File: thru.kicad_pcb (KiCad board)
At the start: 2 copper layers, 33.3 x 12.3 mm, 2 parts, among them J2 Conn_Coaxial, J4 Conn_Coaxial

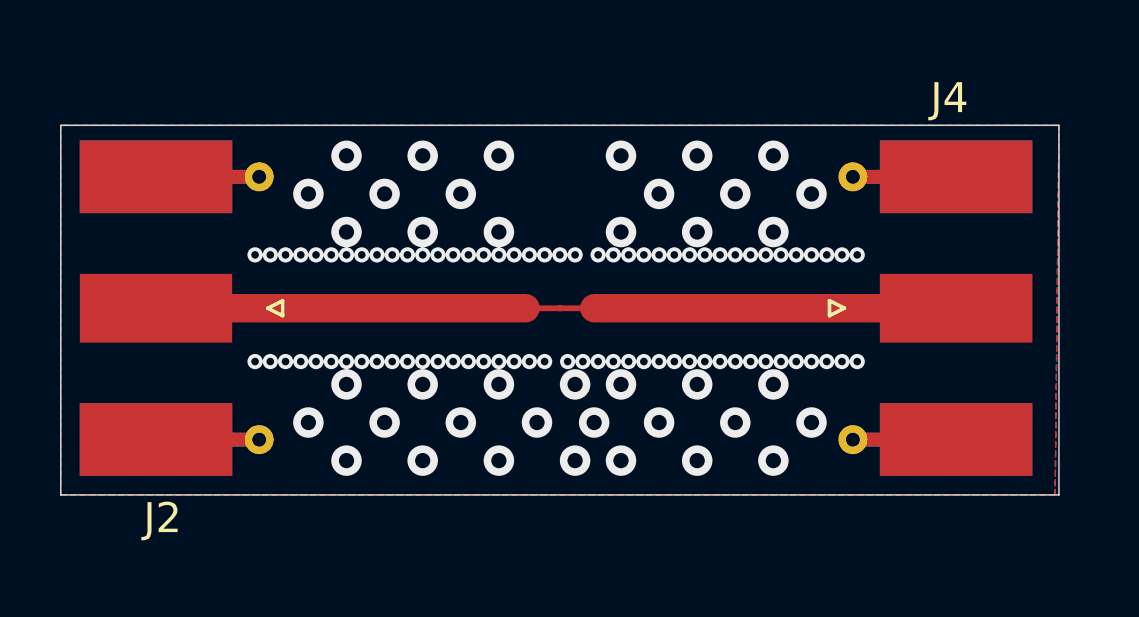
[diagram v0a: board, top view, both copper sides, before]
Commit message: made a southwest microwave launch and put it in the thru
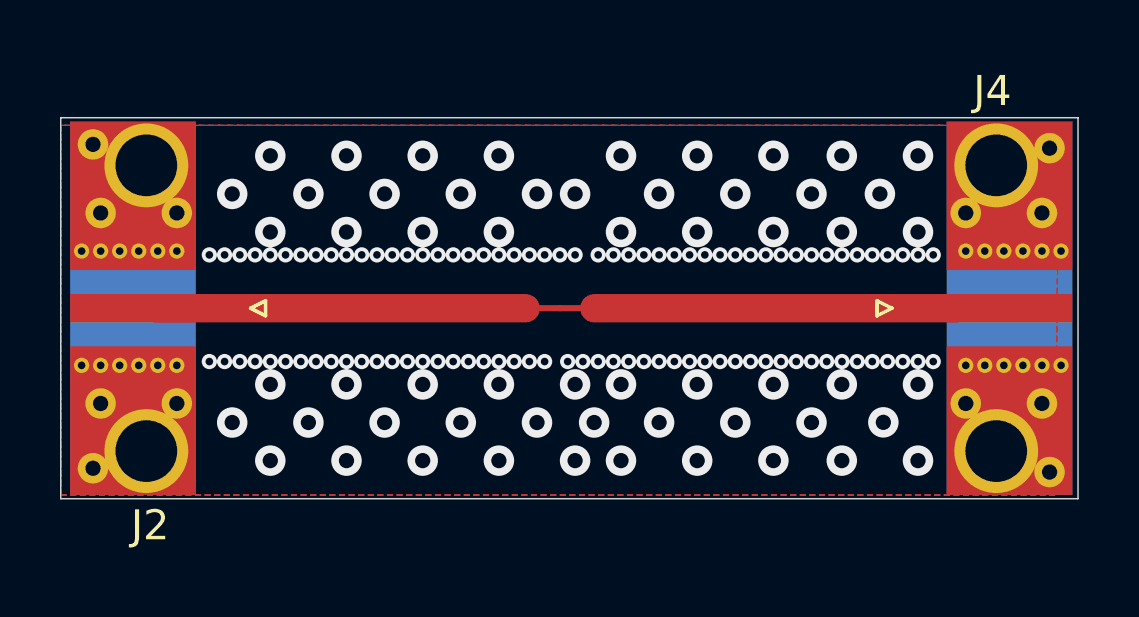
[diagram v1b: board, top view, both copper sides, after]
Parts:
- J2, J4: footprint Connector_Coaxial:SMA_Molex_73251-1153_EdgeMount_Horizontal -> southwest-microwave-connectors:southwest-super-SMA-292-04A-12
- moved J4 5.85 mm to (184.0, 125.4)
- moved J2 4.84 mm to (150.1, 125.4)
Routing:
- net GND: vias 120 -> 154
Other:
- board size 33.3 x 12.3 mm -> 33.9 x 12.7 mm
